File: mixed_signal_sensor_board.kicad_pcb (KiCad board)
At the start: 4 copper layers, 112.5 x 77.5 mm, 154 parts, among them J1 Conn_01x02, J10 Conn_01x04, J11 Conn_01x04, J12 USB_C_Receptacle_USB2.0_16P, J13 Conn_01x04, J14 PYRO, J15 PYRO, J16 PYRO, J17 PYRO, J2 Conn_01x04, J3 Conn_01x06, J4 Conn_01x04, J5 Conn_01x04, J6 Conn_01x04, J7 Conn_01x04, J8 Conn_01x04, J9 Conn_01x04, Q1 Q_NMOS_GDS, Q2 Q_NMOS_GDS, Q3 Q_NMOS_GDS, Q4 Q_NMOS_GDS, SW1 SW_Push, SW2 SW_Push, U1 TMP117xxDRV, U2 LM27762, U3 MagI3C_171013201, U4 TPS7A20xxxDBV, U5 TPS7A20xxxDBV, U6 ADS131M08xPBS, U7 STM32L552CEUx, U8 TCAN3414DRBR, Y1 SG-8018CE_8.192M-TJHSA

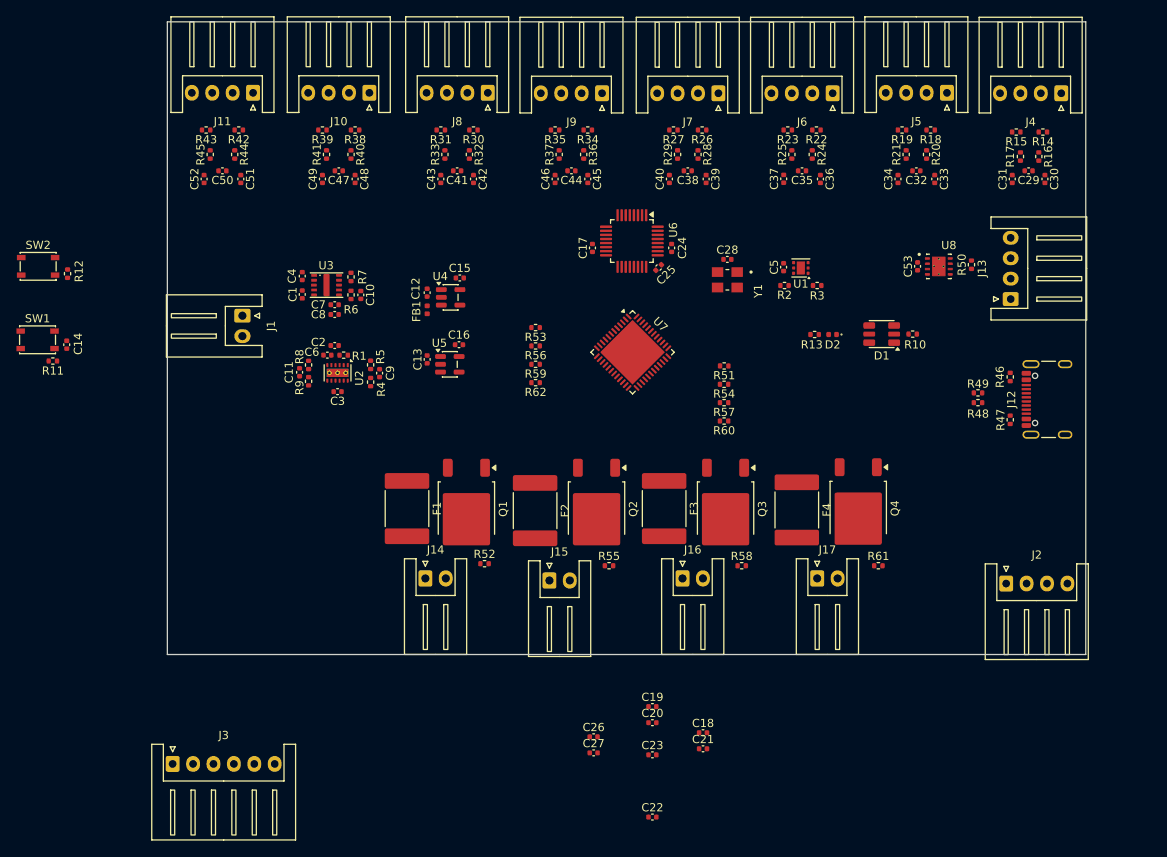
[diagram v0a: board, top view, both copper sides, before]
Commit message: Finished first rough initial layout
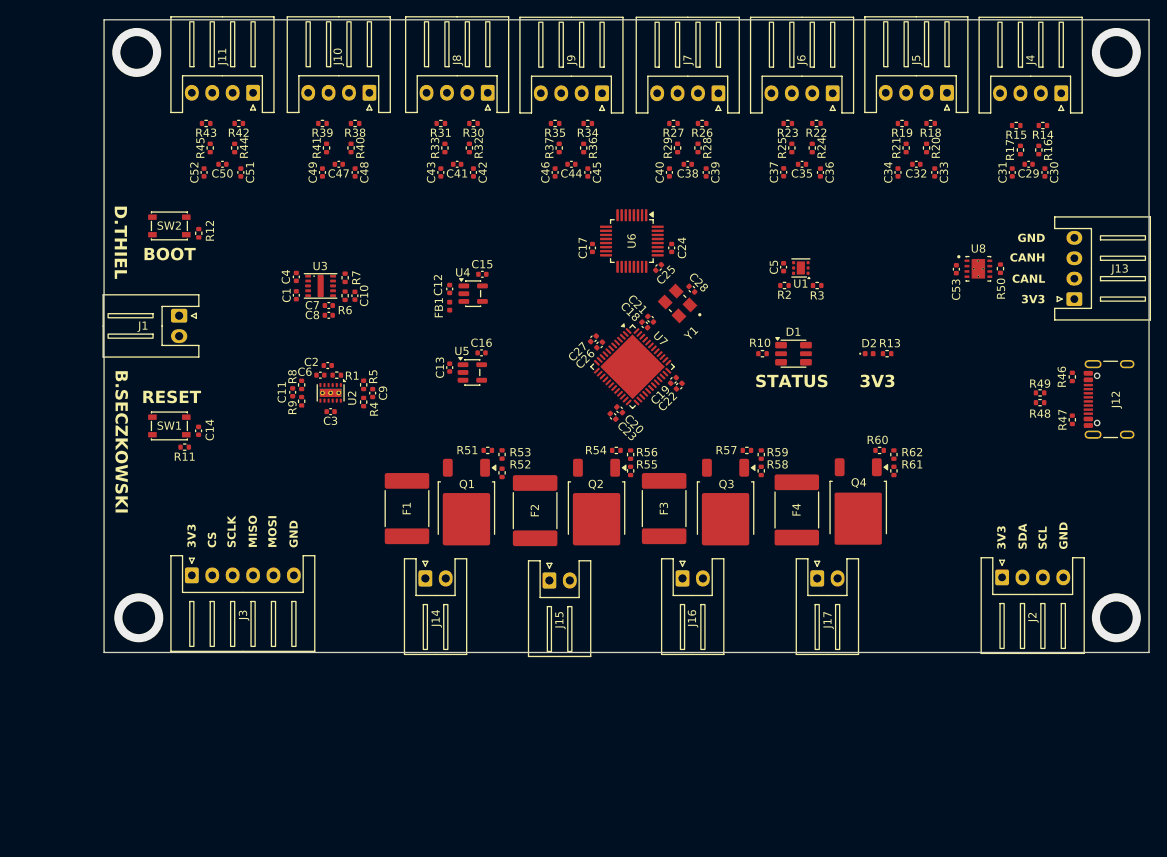
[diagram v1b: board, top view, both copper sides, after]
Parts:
- moved C21 53.0 mm to (159.7, 88.2), turned to 135 degrees
- moved C22 52.9 mm to (163.2, 96.4), turned to 45 degrees
- moved C27 50.7 mm to (152.7, 90.6), turned to -135 degrees
- moved C18 50.5 mm to (159.0, 88.9), turned to 135 degrees
- moved C26 48.0 mm to (153.4, 91.3), turned to -135 degrees
- moved R62 44.8 mm to (189.5, 104.8), turned to 90 degrees
- moved C23 41.7 mm to (155.1, 100.1), turned to -45 degrees
- moved C19 40.0 mm to (162.5, 95.7), turned to 45 degrees
- moved C20 38.5 mm to (155.9, 99.3), turned to -45 degrees
- moved R51 30.8 mm to (139.8, 104.2)
- moved R59 29.8 mm to (173.2, 104.8), turned to 90 degrees
- moved J3 23.2 mm to (103.5, 119.6)
- moved R60 19.4 mm to (187.8, 104.2)
- moved C14 19.3 mm to (104.3, 101.8)
- moved R11 19.3 mm to (102.6, 103.8)
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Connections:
- U7 pad 10: /PYRO1_FAULT -> /ADS_DRDY
- U7 pad 11: /PYRO2_FAULT -> /ADS_SYNC/RESET
- U7 pad 12: /PYRO3_FAULT -> unconnected-(U7-PA2-Pad12)
- U7 pad 13: /PYRO4_FAULT -> unconnected-(U7-PA3-Pad13)
- U7 pad 18: /LEDB -> /PYRO1_SIGNAL
- U7 pad 19: /LEDG -> /PYRO1_FAULT
- U7 pad 20: /LEDR -> /PYRO2_SIGNAL
- U7 pad 21: unconnected-(U7-PB10-Pad21) -> /PYRO2_FAULT
- U7 pad 25: /PYRO1_SIGNAL -> unconnected-(U7-PB12-Pad25)
- U7 pad 26: /PYRO2_SIGNAL -> unconnected-(U7-PB13-Pad26)
- U7 pad 27: /PYRO3_SIGNAL -> unconnected-(U7-PB14-Pad27)
- U7 pad 28: /PYRO4_SIGNAL -> /PYRO3_FAULT
- U7 pad 29: unconnected-(U7-PA8-Pad29) -> /PYRO3_SIGNAL
- U7 pad 30: unconnected-(U7-PA9-Pad30) -> /PYRO4_FAULT
- U7 pad 31: unconnected-(U7-PA10-Pad31) -> /PYRO4_SIGNAL
- U7 pad 39: unconnected-(U7-PB3-Pad39) -> /LEDG
- U7 pad 40: unconnected-(U7-PB4-Pad40) -> /LEDR
- U7 pad 41: unconnected-(U7-PB5-Pad41) -> /LEDB
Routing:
- net (no net): vias 0 -> 4
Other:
- board size 112.5 x 77.5 mm -> 128 x 77.5 mm
- board text added: "3V3"
- board text added: "B.SECZKOWSKI"
- board text added: "BOOT"
- board text added: "CANH"
- board text added: "CANL"
- board text added: "CS"
- board text added: "D.THIEL"
- board text added: "GND"
- board text added: "MISO"
- board text added: "MOSI"
- board text added: "RESET"
- board text added: "SCL"
- board text added: "SCLK"
- board text added: "SDA"
- board text added: "STATUS"
